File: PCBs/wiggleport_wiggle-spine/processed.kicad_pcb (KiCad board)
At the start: 2 copper layers, 88.9 x 114.3 mm, 190 parts, among them CON1 USB-B, CON2 XLR-3 Female, CON3 USB-A, CON4 2.5mm 5-24V 5A, CON5 5-24V 16A, CON6 PLR135, CON7 PLT133, Q1 DMN3190LDW, Q2 2N7002P, Q3 AOD4189, T1 10/100baseT transformer, U1 93C56, U10 SiP32408, U11 SiP32408, U12 TCR2EF25, U13 TCR2EF12, U14 Si5351B, U2 FT2232H, U3 NC7WZ14, U4 AP2204K-5.0, U5 ST485E, U6 iCE40-HX1K-TQ144, U7 RT8299A, U8 RT8299A, U9 SiP32408, X1 12 MHz, X2 25.0000 MHz 15ppm 8pF

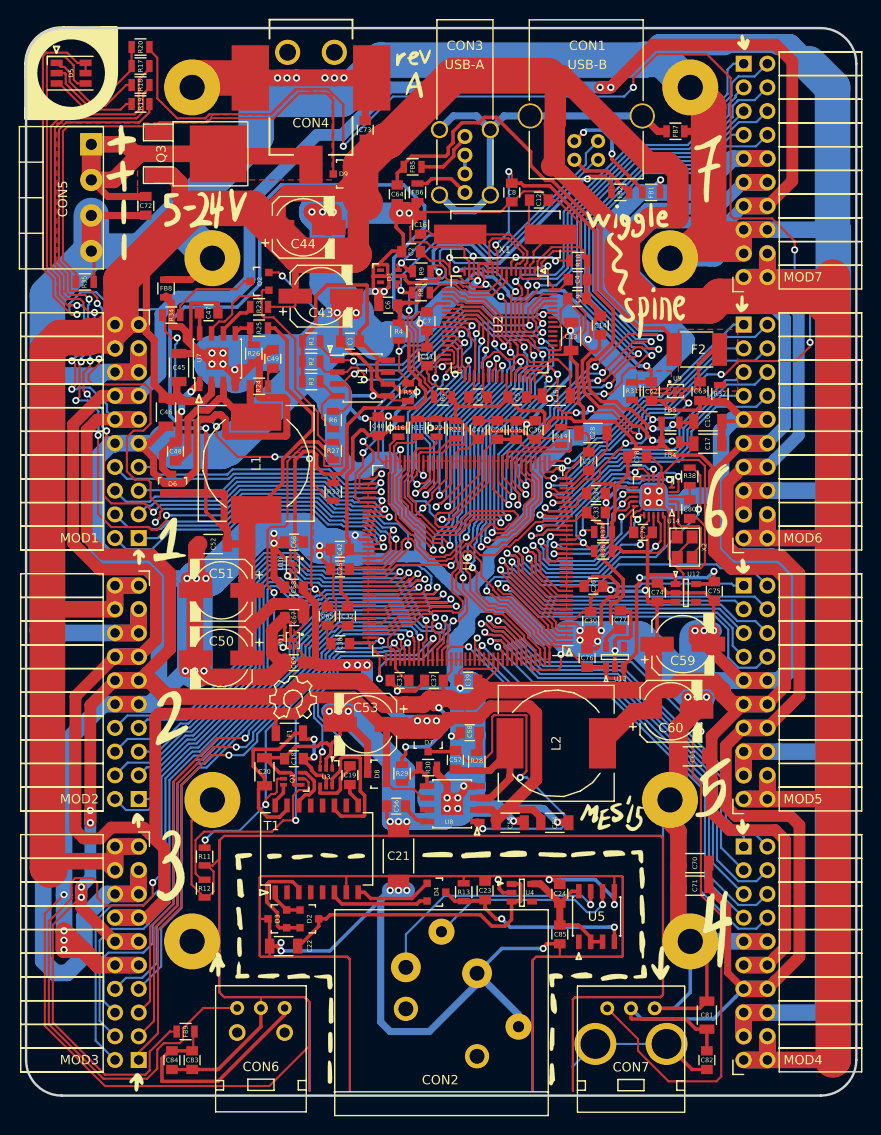
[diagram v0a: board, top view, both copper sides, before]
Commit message: clean psbc that are missed before
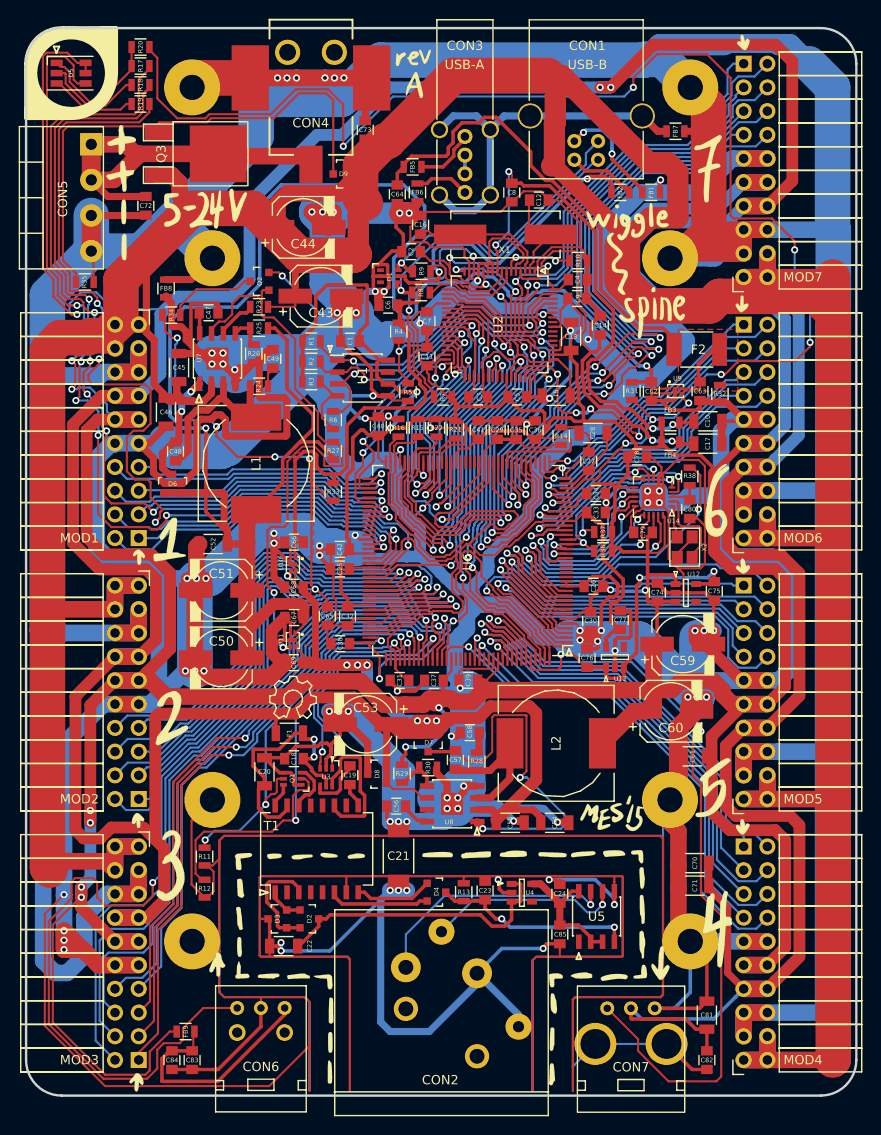
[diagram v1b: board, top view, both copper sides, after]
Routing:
- removed copper zone on F.Cu, net +1V2
- removed copper zone on F.Cu, net +3V3
- removed copper zone on F.Cu, net /Power/5-24V Power Input/POWER_IN
